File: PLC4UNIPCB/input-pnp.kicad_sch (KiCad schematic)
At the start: 3 parts

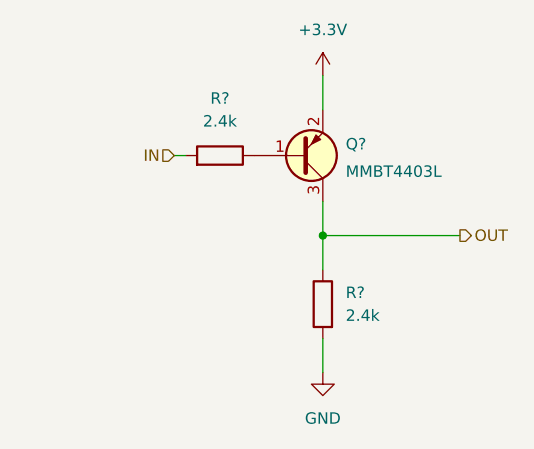
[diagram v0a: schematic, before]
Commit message: Add files via upload
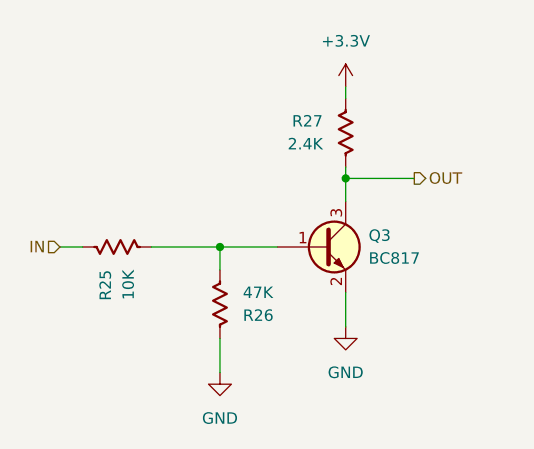
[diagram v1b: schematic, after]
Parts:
- removed Q?: 2SA2018, Package_TO_SOT_SMD_AKL:SOT-416, symbol Transistor_BJT_AKL:2SA2018
- removed R? (x2): 2.4k, Resistor_SMD_AKL:R_0603_1608Metric, symbol Resistor_AKL:R_0603
- added Q3: BC817, PCM_Package_TO_SOT_SMD_AKL:SOT-23, symbol PCM_Transistor_BJT_AKL:BC817
- added R25: 10K, PCM_Resistor_SMD_AKL:R_0603_1608Metric, symbol GP8211S-TC50:R_0603
- added R26: 47K, PCM_Resistor_SMD_AKL:R_0603_1608Metric, symbol GP8211S-TC50:R_0603
- added R27: 2.4K, PCM_Resistor_SMD_AKL:R_0603_1608Metric, symbol GP8211S-TC50:R_0603
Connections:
- net +3.3V: now also R27.2
- net GND: now also Q3.2 (E), R26.2
- net IN: now also R25.2
- net OUT: now also Q3.3 (C), R27.1
- new net: Q3.1 (B), R25.1, R26.1
